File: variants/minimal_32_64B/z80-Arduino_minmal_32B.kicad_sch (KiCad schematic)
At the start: 26 parts, among them SW1 SW_Push, SW3 SW_Push, U1 Z80CPU, U2 74HC373 (74HC573), U3 8282

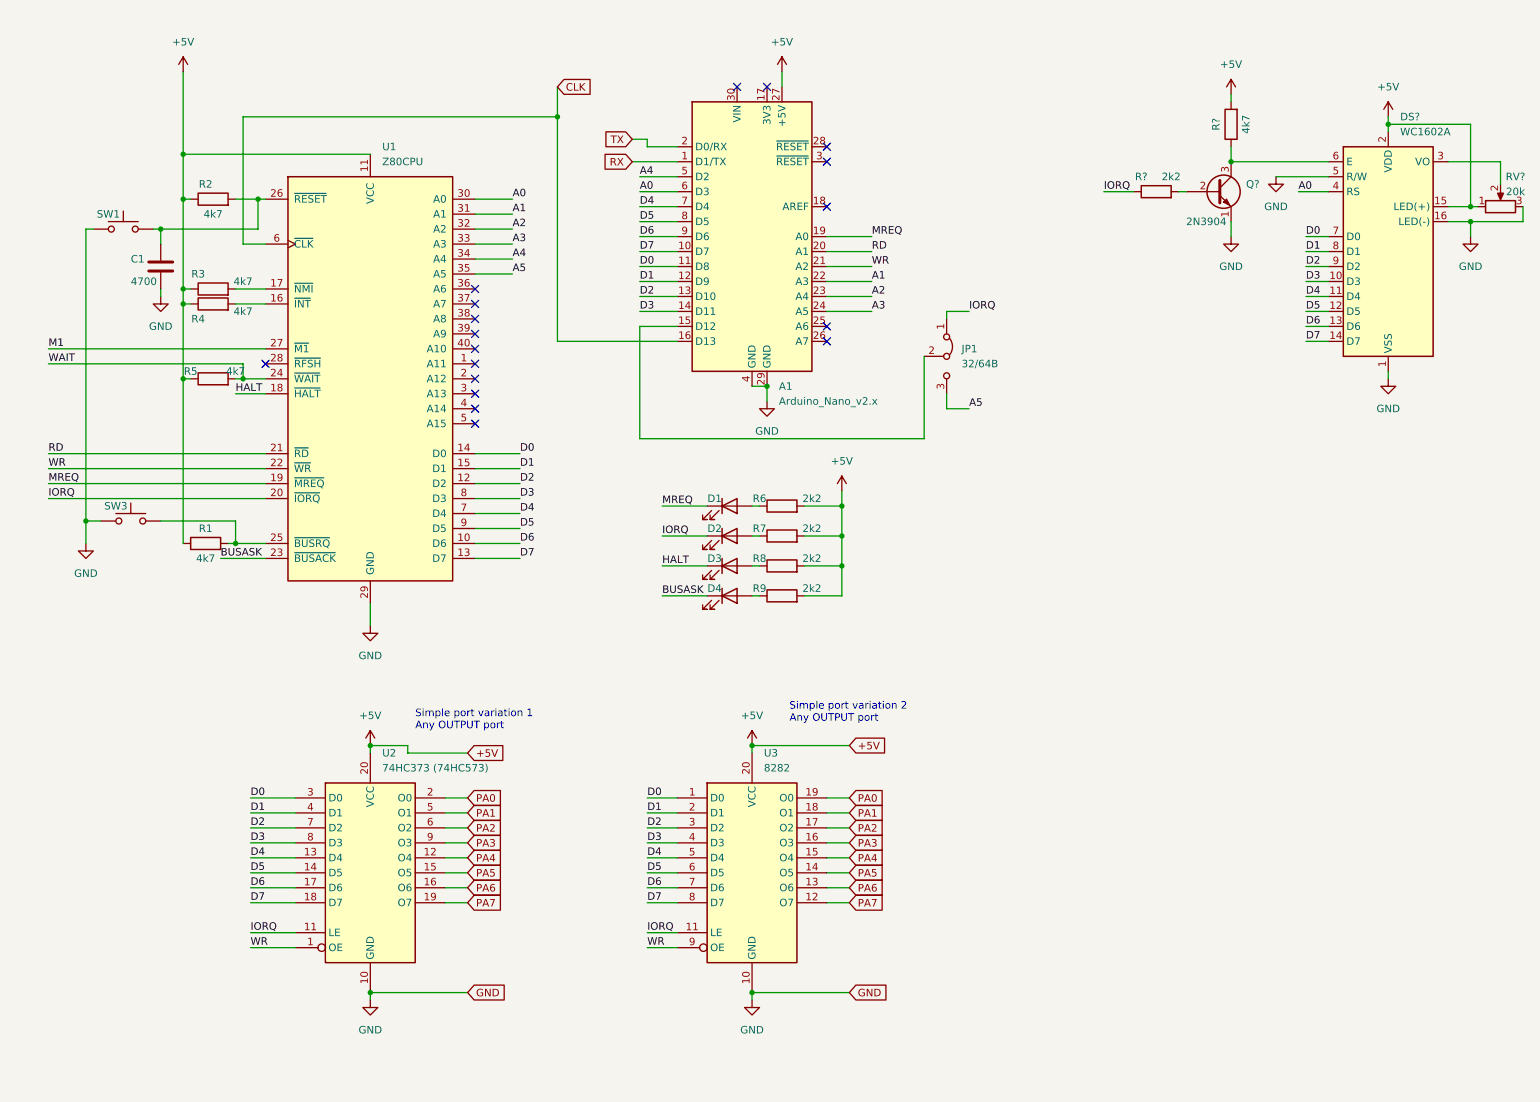
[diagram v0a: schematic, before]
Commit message: Fix changes before IDDLE
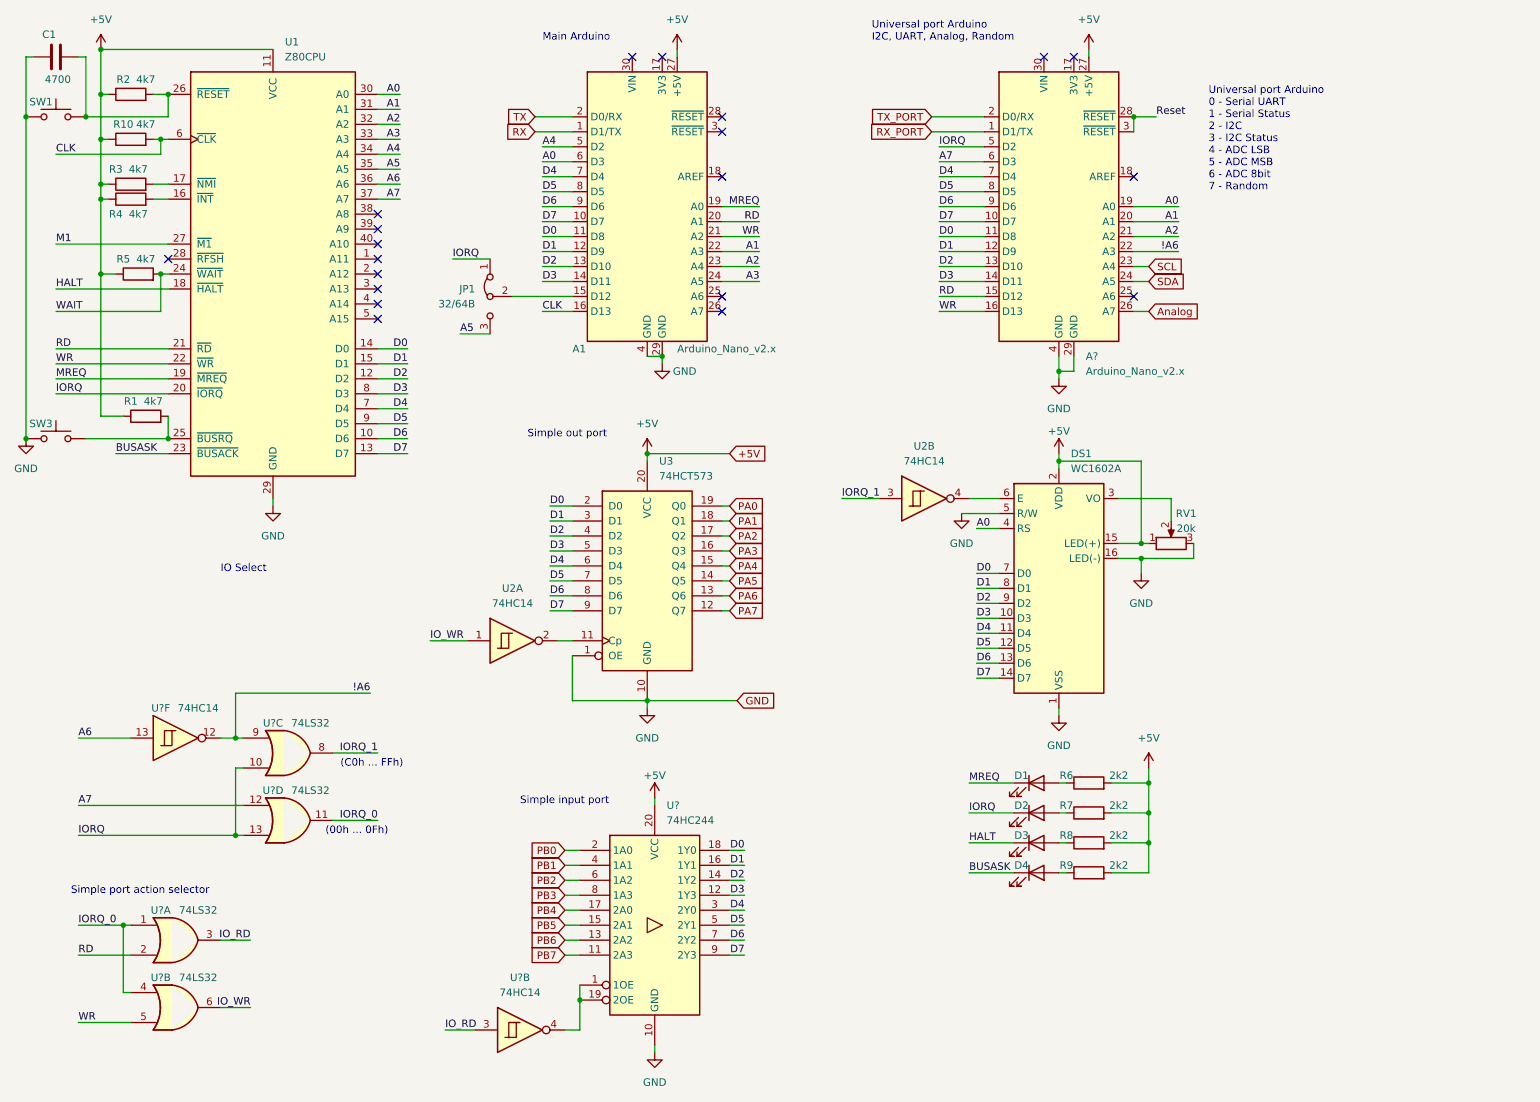
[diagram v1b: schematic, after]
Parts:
- removed Q?: 2N3904, Package_TO_SOT_THT:TO-92_Inline, symbol Transistor_BJT:2N3904
- removed R?: 2k2, symbol Device:R
- removed R?: 4k7, symbol Device:R
- removed U2: 74HC373 (74HC573), symbol 74xx:74HC373
- removed U3: 8282, symbol Custom_components:8282
- added A?: Arduino_Nano_v2.x, Module:Arduino_Nano, symbol MCU_Module:Arduino_Nano_v2.x
- added R10: 4k7, symbol Device:R
- added U2, U? (x2): 74HC14, symbol 74xx:74HC14
- added U3: 74HCT573, symbol 74xx:74HCT574
- added U? (x4): 74LS32, symbol 74xx:74LS32
- added U?: 74HC244, symbol 74xx:74HC244
- gave numbers to parts that had none: 2
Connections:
- net +5V: now also A?.27 (+5V), R10.1, U3.20 (VCC), U?.20 (VCC)
- net A0: now also A?.19 (A0)
- net A1: now also A?.20 (A1)
- net A2: now also A?.21 (A2)
- net CLK: now also R10.2
- net D0: now also A?.11 (D8), U3.2 (D0), U?.18 (1Y0)
- net D1: now also A?.12 (D9), U3.3 (D1), U?.16 (1Y1)
- net D2: now also A?.13 (D10), U3.4 (D2), U?.14 (1Y2)
- net D3: now also A?.14 (D11), U3.5 (D3), U?.12 (1Y3)
- net D4: now also A?.7 (D4), U3.6 (D4), U?.3 (2Y0)
- net D5: now also A?.8 (D5), U3.7 (D5), U?.5 (2Y1)
- net D6: now also A?.9 (D6), U3.8 (D6), U?.7 (2Y2)
- net D7: now also A?.10 (D7), U3.9 (D7), U?.9 (2Y3)
- net GND: now also C1.1, A?.29 (GND), A?.4 (GND), U3.1 (OE), U3.10 (GND), U?.10 (GND); no longer C1.2
- net IORQ: now also A?.5 (D2), U?.10, U?.13
- net PA0: now also U3.19 (Q0)
- net PA1: now also U3.18 (Q1)
- net PA2: now also U3.17 (Q2)
- net PA3: now also U3.16 (Q3)
- net PA4: now also U3.15 (Q4)
- net PA5: now also U3.14 (Q5)
- net PA6: now also U3.13 (Q6)
- net PA7: now also U3.12 (Q7)
- net RD: now also A?.15 (D12), U?.2
- net WR: now also A?.16 (D13), U?.5
- net at DS1.6 (E): now also U2.4
- net at R2.2, SW1.2, U1.26 (~{RESET}): now also C1.2; no longer C1.1
- net A6: now reaches U1.36 (A6)
- net A6: now also U?.13
- net A7: now reaches U1.37 (A7)
- net A7: now also A?.6 (D3), U?.12
- new net: U?.1 (1OE), U?.19 (2OE), U?.4
- new net: U2.2, U3.11 (Cp)
- new net !A6: A?.22 (A3), U?.12, U?.9
- new net Analog: A?.26 (A7)
- new net IORQ_0: U?.1, U?.11, U?.4
- new net IORQ_1: U2.3, U?.8
- new net IO_RD: U?.3, U?.3
- new net IO_WR: U2.1, U?.6
- new net PB0: U?.2 (1A0)
- new net PB1: U?.4 (1A1)
- new net PB2: U?.6 (1A2)
- new net PB3: U?.8 (1A3)
- new net PB4: U?.17 (2A0)
- new net PB5: U?.15 (2A1)
- new net PB6: U?.13 (2A2)
- new net PB7: U?.11 (2A3)
- new net RX_PORT: A?.1 (D1/TX)
- new net Reset: A?.28 (~{RESET}), A?.3 (~{RESET})
- new net SCL: A?.23 (A4)
- new net SDA: A?.24 (A5)
- new net TX_PORT: A?.2 (D0/RX)
- no-connect marks 18 -> 20
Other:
- note added: "(00h ... 0Fh)"
- note added: "(C0h ... FFh)"
- note added: "IO Select"
- note added: "Main Arduino"
- note added: "Simple input port"
- note added: "Simple out port"
- note added: "Simple port action selector"
- note added: "Universal port Arduino 0 - Serial UART 1 - Serial Status 2 - I2C 3 - I2C Status 4 - ADC LSB 5 - ADC MSB 6 - ADC 8bit 7 - Random"
- note added: "Universal port Arduino I2C, UART, Analog, Random"
- note removed: "Simple port variation 1 Any OUTPUT port"
- note removed: "Simple port variation 2 Any OUTPUT port"
- moved on the sheet: A1, C1, D1, D2, D3, D4, DS1, JP1, R2, R3, R4, R5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
